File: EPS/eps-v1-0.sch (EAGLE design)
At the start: 84 parts, among them IC1 MIC79110, IC10 MAX4374-10UMAX, IC11 TLV70228DBV, IC2 MIC79110, IC3 LT3872, IC4 LT3872, IC5 INA291-D, IC6 NCS2202, IC7 NCS2202, IC8 TLV70233DBVR, IC9 AD7998, Q1 SI7448DP, Q2 SI7448DP, Q3 SI7448DP, Q4 SI7485DP, Q6 SI7485DP, Q8 SI7485DP, Q9 SI7448DP

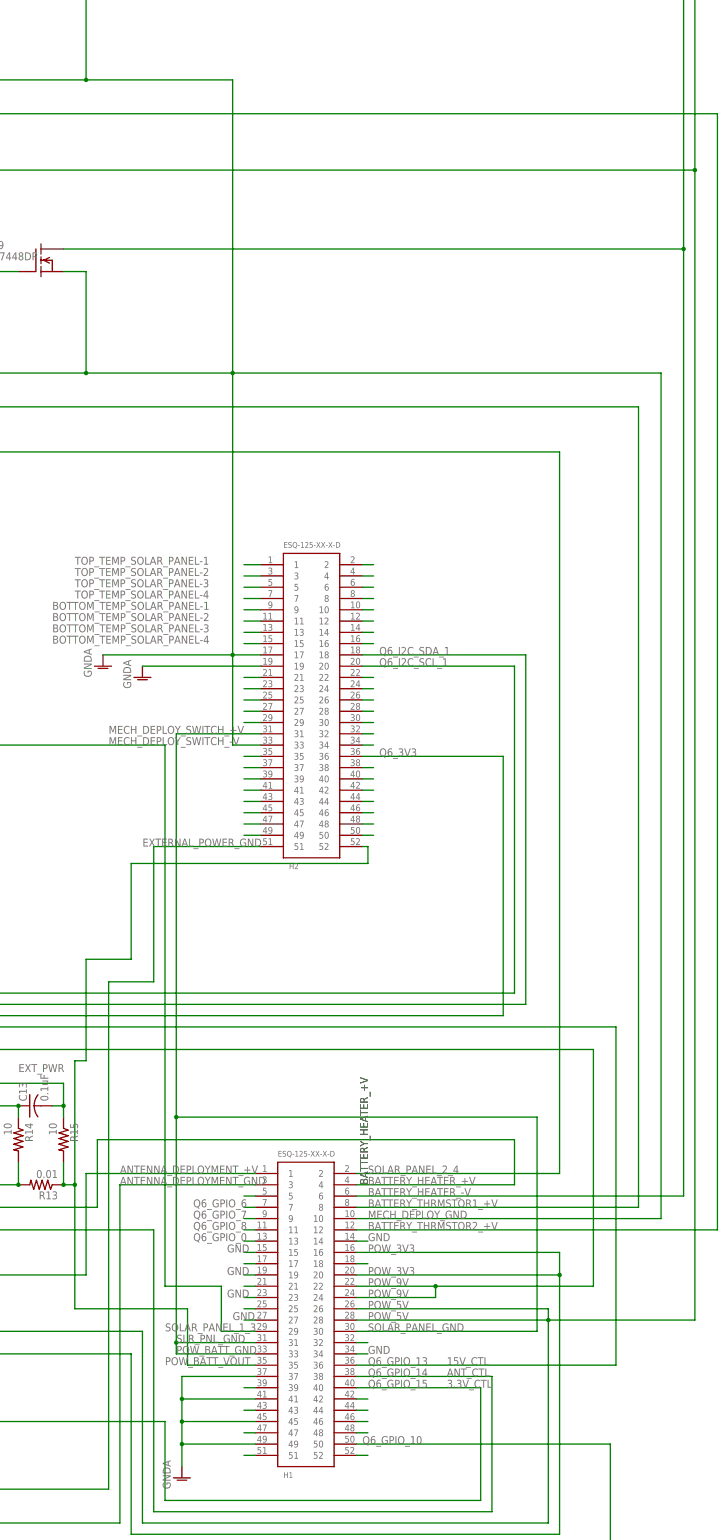
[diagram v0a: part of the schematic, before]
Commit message: Revert "Fixed all the trivial wiring issues for the CDH, Diplexer, EPS and wiring harness schematics"
This reverts commits
  6713d85a6277b26f983fd7a52d0f95a7f9e4e046.
  086194ae58682b6763f31692a26cd4dac33df983
  82b42737f0fe6cd82dfea4a4ae7507beb01cc7b8

This revert is required because changing/connecting net names in eagle will automatically modify or destroy PCB traces associated with those netnames.
Updating the schematics and PCBs will need to be redone carefully to ensure no traces are destroyed.

	modified:   CDH-V3.7/CDH-v3.7.brd
	modified:   CDH-V3.7/CDH-v3.7.sch
	modified:   Diplexer/diplexer_v4rev0-schematic.sch
	modified:   EPS/eps-v1-0.brd
	modified:   EPS/eps-v1-0.sch
	modified:   Payload Internal - Auxiliary/Payload v2.1.brd
	modified:   Payload Internal - Auxiliary/Payload v2.1.sch
	modified:   Wiring Harness/wiring-harness-complete-v1.0.sch
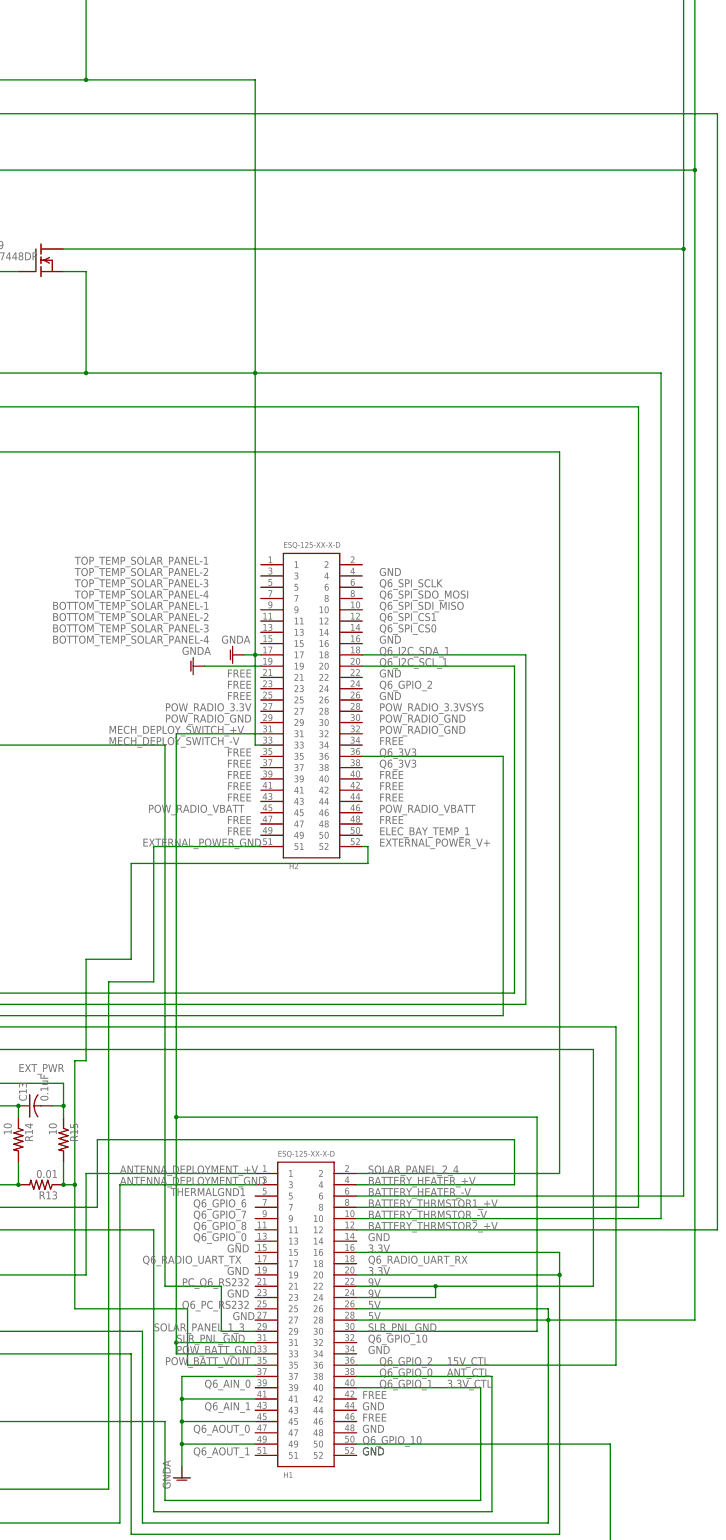
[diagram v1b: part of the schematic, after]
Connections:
- net ANTENNA_DEPLOYMENT_+V renamed N$12
- net BATTERY_HEATER_+V renamed N$43
- net BATTERY_HEATER_-V renamed N$4
- net BATTERY_THRMSTOR1_+V renamed N$50
- net BATTERY_THRMSTOR2_+V renamed N$2
- net POW_3V3 renamed N$44
- net POW_5V renamed N$18
- net POW_9V renamed N$11
- net POW_BATT_VOUT renamed N$46
- net Q6_GPIO_13 renamed N$5
- net Q6_GPIO_14 renamed N$36
- net Q6_GPIO_15 renamed N$13
- net Q6_I2C_SCL_1 renamed N$42
- net Q6_I2C_SDA_1 renamed N$41
- net SOLAR_PANEL_1_3 renamed N$34
- net SOLAR_PANEL_2_4 renamed N$15
- net SOLAR_PANEL_GND renamed N$22
- removed net +3V3: C14.1, C19.1, C20.1, H2.36, H2.38, IC5.VS, IC9.VDD@2, IC9.VDD@5, IC9.VREF_IN, R38.2
- removed net BOTTOM_TEMP_SOLAR_PANEL-1: H2.9
- removed net BOTTOM_TEMP_SOLAR_PANEL-2: H2.11
- removed net BOTTOM_TEMP_SOLAR_PANEL-3: H2.13
- removed net BOTTOM_TEMP_SOLAR_PANEL-4: H2.15
- removed net ELEC_BAY_TEMP_1: H2.50
- removed net GND: H1.15, H1.19, H1.23, H1.27, H1.34, H1.44, H1.48, H1.52, H2.16, H2.22, H2.26, H2.4
- removed net MECH_DEPLOY_GND: C15.2, C16.2, H1.10, H2.17, H2.33, IC6.VEE, IC7.VEE, Q3.S, Q9.S, R10.1, R27.1
- removed net N$1 (its old number): H2.6
- removed net N$11 (its old number): H2.2
- removed net N$13 (its old number): H2.49
- removed net N$15 (its old number): H2.47
- removed net N$17 (its old number): H2.14
- removed net N$2 (its old number): H1.42
- removed net N$22 (its old number): H2.34
- removed net N$27 (its old number): H2.44
- removed net N$4 (its old number): H2.8
- removed net N$5 (its old number): H2.48
- removed net N$6: H2.10
- removed net N$654643543: H1.14
- removed net N$78: H2.39
- removed net N$79: H2.41
- removed net N$80: H2.43
- removed net N$81: H2.40
- removed net N$82: H2.42
- removed net N$83: H1.46
- removed net N$9 (its old number): H2.12
- removed net PC_Q6_RS232: H1.21
- removed net POW_RADIO_3V3: H2.27
- removed net POW_RADIO_3V3_SYS: H2.28
- removed net POW_RADIO_GND: H2.29, H2.30, H2.32
- removed net POW_RADIO_VBATT: H2.45, H2.46
- removed net Q6_AIN_0: H1.39
- removed net Q6_AIN_1: H1.43
- removed net Q6_AOUT_0: H1.47
- removed net Q6_AOUT_1: H1.51
- removed net Q6_GPIO_0: H1.13
- removed net Q6_GPIO_10: H1.32, H1.50, IC10.COT1, R38.1
- removed net Q6_GPIO_2: H2.24
- removed net Q6_GPIO_6: H1.7
- removed net Q6_GPIO_7: H1.9
- removed net Q6_GPIO_8: H1.11
- removed net Q6_PC_RS232: H1.25
- removed net Q6_RADIO_UART_RX: H1.18
- removed net Q6_RADIO_UART_TX: H1.17
- removed net Q6_SPI_CS0: H2.37
- removed net Q6_SPI_CS1: H2.25
- removed net Q6_SPI_SCLK: H2.21
- removed net Q6_SPI_SDI_MISO: H2.35
- removed net Q6_SPI_SDO_MOSI: H2.23
- removed net THERMALGND1: H1.5
- removed net TOP_TEMP_SOLAR_PANEL-1: H2.1
- removed net TOP_TEMP_SOLAR_PANEL-2: H2.3
- removed net TOP_TEMP_SOLAR_PANEL-3: H2.5
- removed net TOP_TEMP_SOLAR_PANEL-4: H2.7
- new net N$49: H1.50, IC10.COT1, R38.1
- new net N$58: C14.1, C19.1, C20.1, H2.36, IC5.VS, IC9.VDD@2, IC9.VDD@5, IC9.VREF_IN, R38.2
- net GNDA: now also C15.2, C16.2, H1.10, H2.17, H2.33, IC6.VEE, IC7.VEE, Q3.S, Q9.S, R10.1, R27.1
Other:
- note added: "9V"
- note added: "BATTERY_HEATER_+V"
- note added: "BATTERY_HEATER_-V"
- note added: "BATTERY_THRMSTOR1_+V"
- note added: "BATTERY_THRMSTOR2_+V"
- note added: "BATTERY_THRMSTOR_-V"
- note added: "ELEC_BAY_TEMP_1"
- note added: "EXTERNAL_POWER_V+"
- note added: "FREE"
- note added: "PC_Q6_RS232"
- note added: "POW_RADIO_3.3V"
- note added: "POW_RADIO_3.3VSYS"
- note added: "POW_RADIO_GND"
- note added: "POW_RADIO_VBATT"
- note added: "Q6_AIN_0"
- note added: "Q6_AIN_1"
- note added: "Q6_AOUT_0"
- note added: "Q6_AOUT_1"
- note added: "Q6_GPIO_1"
- note added: "Q6_GPIO_2"
- note added: "Q6_I2C_SCL_1"
- note added: "Q6_I2C_SDA_1"
- note added: "Q6_PC_RS232"
- note added: "Q6_RADIO_UART_RX"
- note added: "Q6_RADIO_UART_TX"
- note added: "Q6_SPI_CS0"
- note added: "Q6_SPI_CS1"
- note added: "Q6_SPI_SCLK"
- note added: "Q6_SPI_SDI_MISO"
- note added: "Q6_SPI_SDO_MOSI"
- note added: "THERMALGND1"

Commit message: Fixed all the trivial wiring issues for the CDH, Diplexer, EPS and wiring harness schematics
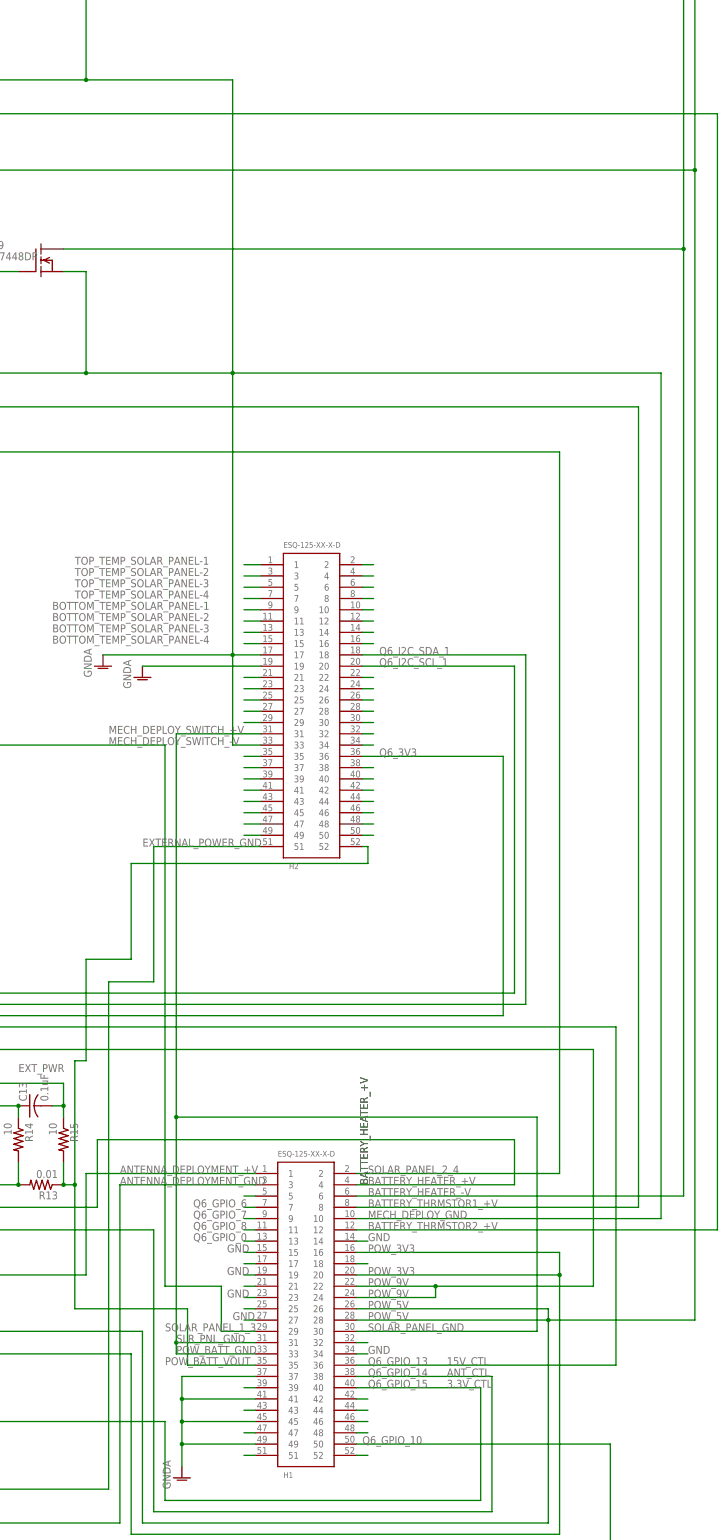
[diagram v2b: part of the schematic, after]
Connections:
- net N$11 renamed POW_9V
- net N$12 renamed ANTENNA_DEPLOYMENT_+V
- net N$13 renamed Q6_GPIO_15
- net N$15 renamed SOLAR_PANEL_2_4
- net N$18 renamed POW_5V
- net N$2 renamed BATTERY_THRMSTOR2_+V
- net N$22 renamed SOLAR_PANEL_GND
- net N$34 renamed SOLAR_PANEL_1_3
- net N$36 renamed Q6_GPIO_14
- net N$4 renamed BATTERY_HEATER_-V
- net N$41 renamed Q6_I2C_SDA_1
- net N$42 renamed Q6_I2C_SCL_1
- net N$43 renamed BATTERY_HEATER_+V
- net N$44 renamed POW_3V3
- net N$46 renamed POW_BATT_VOUT
- net N$5 renamed Q6_GPIO_13
- net N$50 renamed BATTERY_THRMSTOR1_+V
- removed net N$58: C14.1, C19.1, C20.1, H2.36, IC5.VS, IC9.VDD@2, IC9.VDD@5, IC9.VREF_IN, R38.2
- new net +3V3: C14.1, C19.1, C20.1, H2.36, H2.38, IC5.VS, IC9.VDD@2, IC9.VDD@5, IC9.VREF_IN, R38.2
- new net BOTTOM_TEMP_SOLAR_PANEL-1: H2.9
- new net BOTTOM_TEMP_SOLAR_PANEL-2: H2.11
- new net BOTTOM_TEMP_SOLAR_PANEL-3: H2.13
- new net BOTTOM_TEMP_SOLAR_PANEL-4: H2.15
- new net ELEC_BAY_TEMP_1: H2.50
- new net GND: H1.15, H1.19, H1.23, H1.27, H1.34, H1.44, H1.48, H1.52, H2.16, H2.22, H2.26, H2.4
- new net MECH_DEPLOY_GND: C15.2, C16.2, H1.10, H2.17, H2.33, IC6.VEE, IC7.VEE, Q3.S, Q9.S, R10.1, R27.1
- new net N$1: H2.6
- new net N$11: H2.2
- new net N$13: H2.49
- new net N$15: H2.47
- new net N$17: H2.14
- new net N$2: H1.42
- new net N$22: H2.34
- new net N$27: H2.44
- new net N$4: H2.8
- new net N$5: H2.48
- new net N$6: H2.10
- new net N$654643543: H1.14
- new net N$78: H2.39
- new net N$79: H2.41
- new net N$80: H2.43
- new net N$81: H2.40
- new net N$82: H2.42
- new net N$83: H1.46
- new net N$9: H2.12
- new net PC_Q6_RS232: H1.21
- new net POW_RADIO_3V3: H2.27
- new net POW_RADIO_3V3_SYS: H2.28
- new net POW_RADIO_GND: H2.29, H2.30, H2.32
- new net POW_RADIO_VBATT: H2.45, H2.46
- new net Q6_AIN_0: H1.39
- new net Q6_AIN_1: H1.43
- new net Q6_AOUT_0: H1.47
- new net Q6_AOUT_1: H1.51
- new net Q6_GPIO_0: H1.13
- new net Q6_GPIO_10: H1.32
- new net Q6_GPIO_2: H2.24
- new net Q6_GPIO_6: H1.7
- new net Q6_GPIO_7: H1.9
- new net Q6_GPIO_8: H1.11
- new net Q6_PC_RS232: H1.25
- new net Q6_RADIO_UART_RX: H1.18
- new net Q6_RADIO_UART_TX: H1.17
- new net Q6_SPI_CS0: H2.37
- new net Q6_SPI_CS1: H2.25
- new net Q6_SPI_SCLK: H2.21
- new net Q6_SPI_SDI_MISO: H2.35
- new net Q6_SPI_SDO_MOSI: H2.23
- new net THERMALGND1: H1.5
- new net TOP_TEMP_SOLAR_PANEL-1: H2.1
- new net TOP_TEMP_SOLAR_PANEL-2: H2.3
- new net TOP_TEMP_SOLAR_PANEL-3: H2.5
- new net TOP_TEMP_SOLAR_PANEL-4: H2.7
- net GNDA: no longer C15.2, C16.2, H1.10, H2.17, H2.33, IC6.VEE, IC7.VEE, Q3.S, Q9.S, R10.1, R27.1
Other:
- note removed: "9V"
- note removed: "BATTERY_HEATER_+V"
- note removed: "BATTERY_HEATER_-V"
- note removed: "BATTERY_THRMSTOR1_+V"
- note removed: "BATTERY_THRMSTOR2_+V"
- note removed: "BATTERY_THRMSTOR_-V"
- note removed: "ELEC_BAY_TEMP_1"
- note removed: "EXTERNAL_POWER_V+"
- note removed: "FREE"
- note removed: "PC_Q6_RS232"
- note removed: "POW_RADIO_3.3V"
- note removed: "POW_RADIO_3.3VSYS"
- note removed: "POW_RADIO_GND"
- note removed: "POW_RADIO_VBATT"
- note removed: "Q6_AIN_0"
- note removed: "Q6_AIN_1"
- note removed: "Q6_AOUT_0"
- note removed: "Q6_AOUT_1"
- note removed: "Q6_GPIO_1"
- note removed: "Q6_GPIO_2"
- note removed: "Q6_I2C_SCL_1"
- note removed: "Q6_I2C_SDA_1"
- note removed: "Q6_PC_RS232"
- note removed: "Q6_RADIO_UART_RX"
- note removed: "Q6_RADIO_UART_TX"
- note removed: "Q6_SPI_CS0"
- note removed: "Q6_SPI_CS1"
- note removed: "Q6_SPI_SCLK"
- note removed: "Q6_SPI_SDI_MISO"
- note removed: "Q6_SPI_SDO_MOSI"
- note removed: "THERMALGND1"
